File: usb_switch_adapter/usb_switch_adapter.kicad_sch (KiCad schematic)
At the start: 10 parts, among them J1 USB-C Plug, J2 USB2.0-C_SMT, SW1 SW_Push, U1 CH217K, U2 CH32V003J4M6

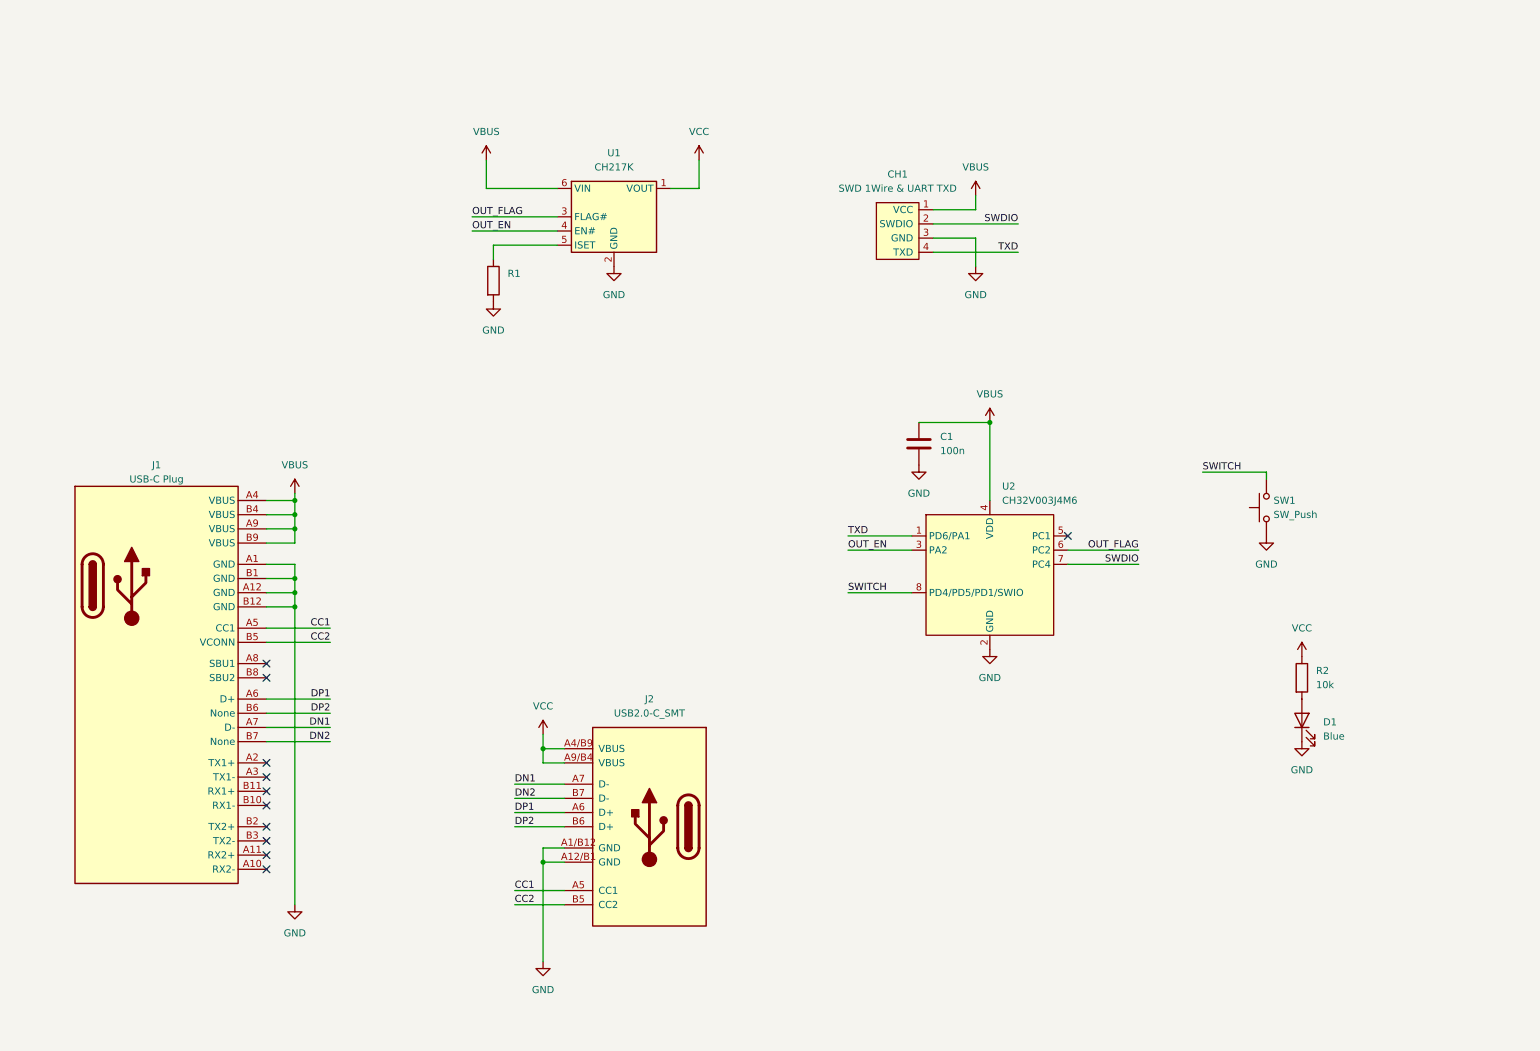
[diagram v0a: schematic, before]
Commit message: usb-switch-adapter/1.0.0
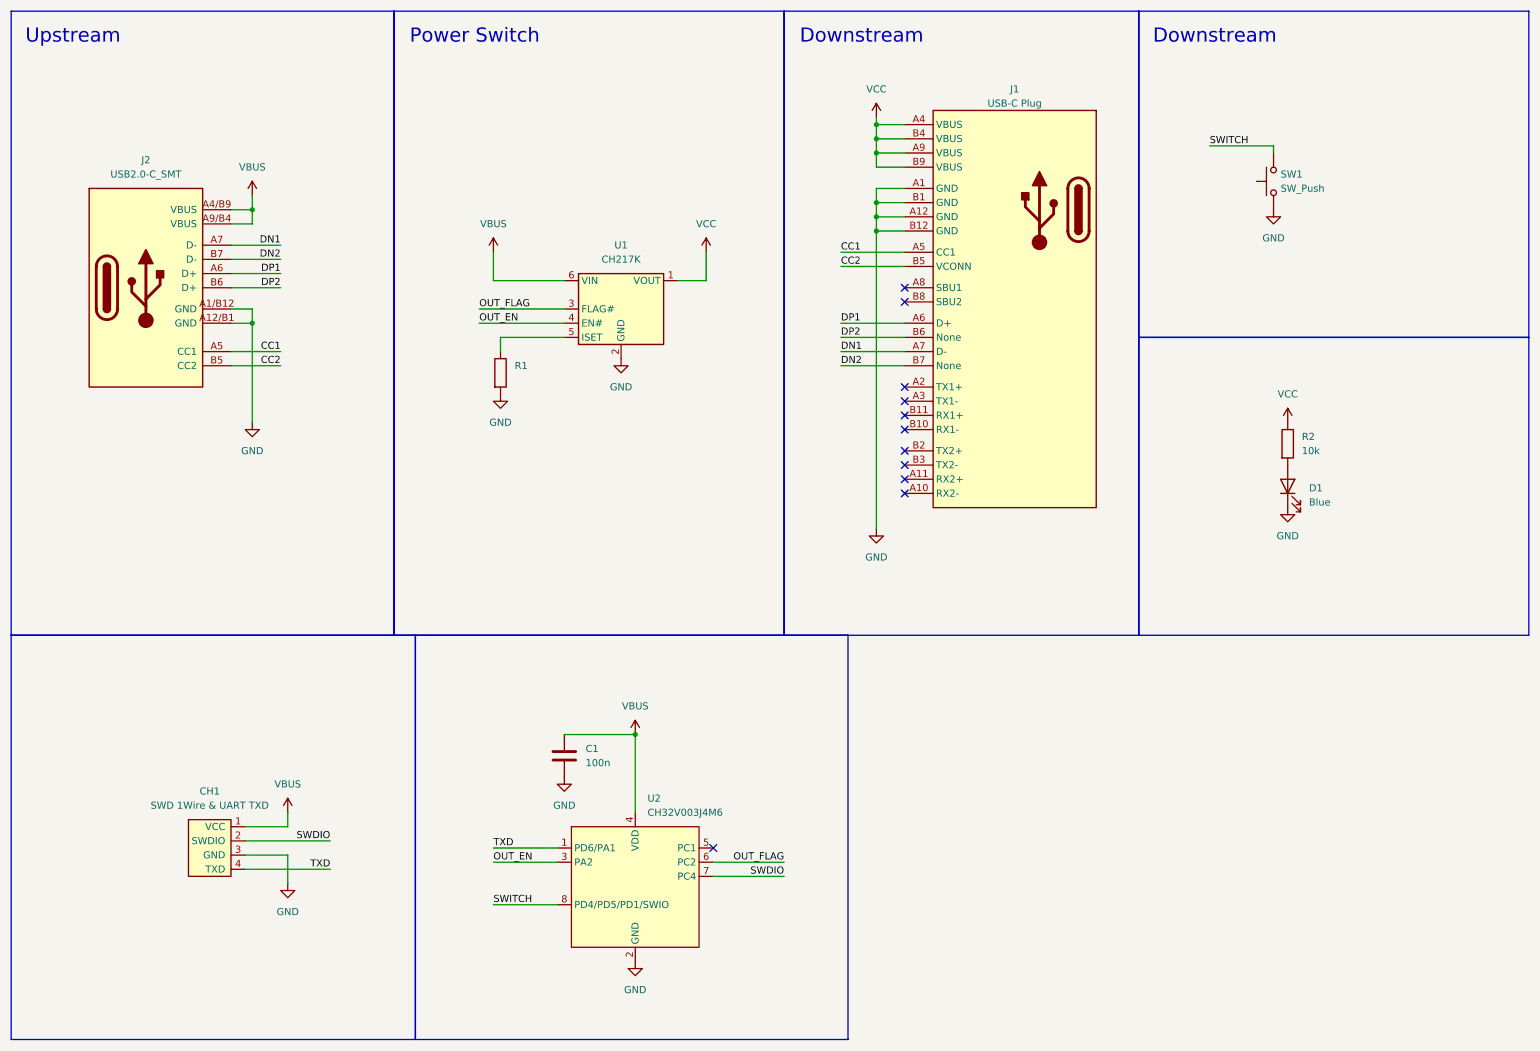
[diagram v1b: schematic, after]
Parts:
- U1: footprint Package_TO_SOT_SMD:SOT-23-6 -> 74th:Package_SOT-23-6
- U2: footprint Package_SO:SOIC-8_3.9x4.9mm_P1.27mm -> 74th:Package_SOIC-8_3.9x4.9mm_P1.27mm
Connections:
- net VBUS: now also J2.A4/B9 (VBUS), J2.A9/B4 (VBUS); no longer J1.A4 (VBUS), J1.A9 (VBUS), J1.B4 (VBUS), J1.B9 (VBUS)
- net VCC: now also J1.A4 (VBUS), J1.A9 (VBUS), J1.B4 (VBUS), J1.B9 (VBUS); no longer J2.A4/B9 (VBUS), J2.A9/B4 (VBUS)
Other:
- note added: "Downstream"
- note added: "Power Switch"
- note added: "Upstream"
- company: (none) -> Atsushi Morimoto (@74th)
- title: (none) -> USB Switch Adapter
- moved on the sheet: C1, CH1, D1, J1, J2, R1, R2, SW1, U1, U2
